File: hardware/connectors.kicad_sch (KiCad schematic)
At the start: 8 parts, among them J1 USB_C_Receptacle_USB2.0_16P, J2 FTSH-107-01-L-D-K, J3 POWER & CAN, J4 PWM1, J5 PWM2, T12 TP_VBUS

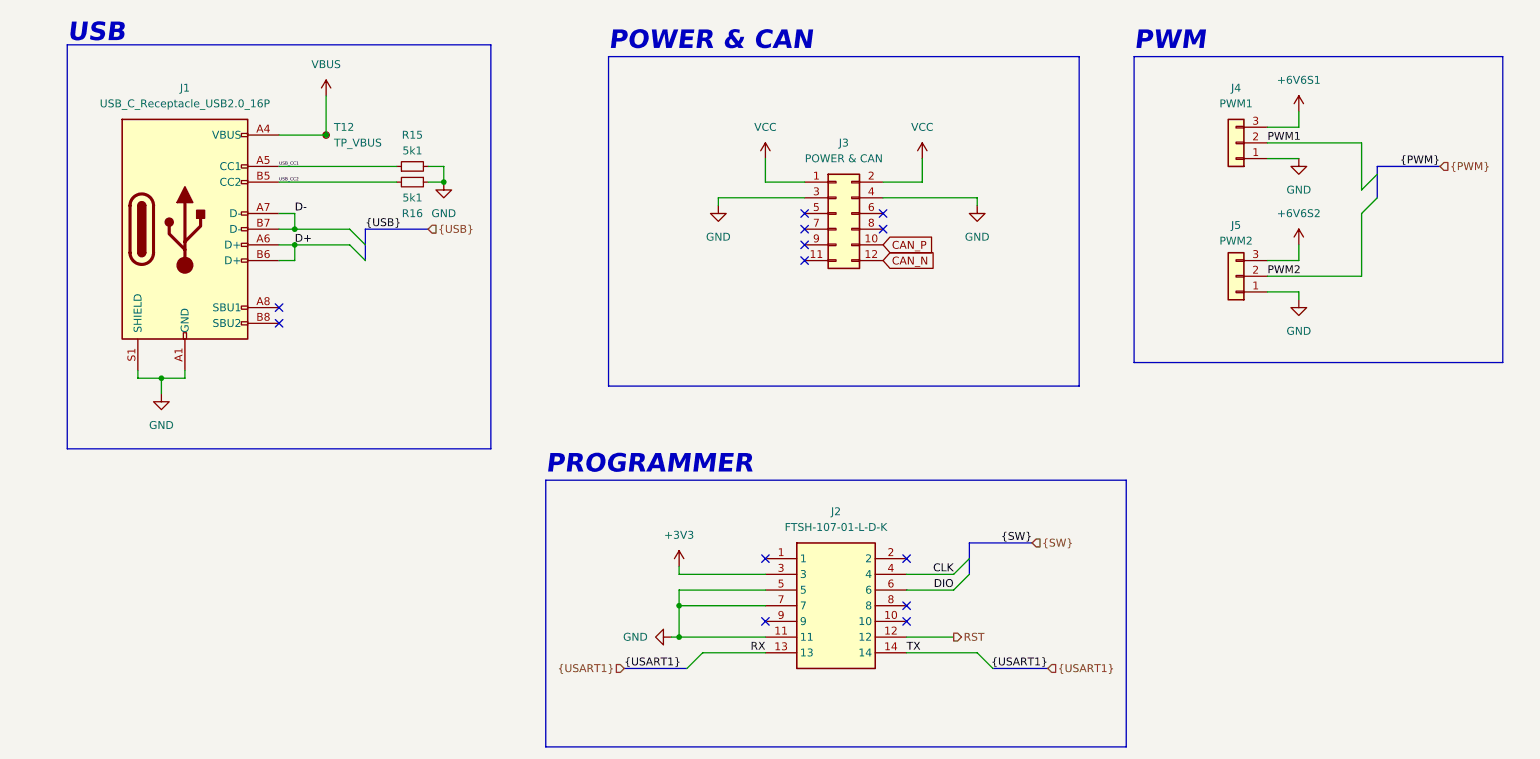
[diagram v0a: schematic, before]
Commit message: pcb & scheme update
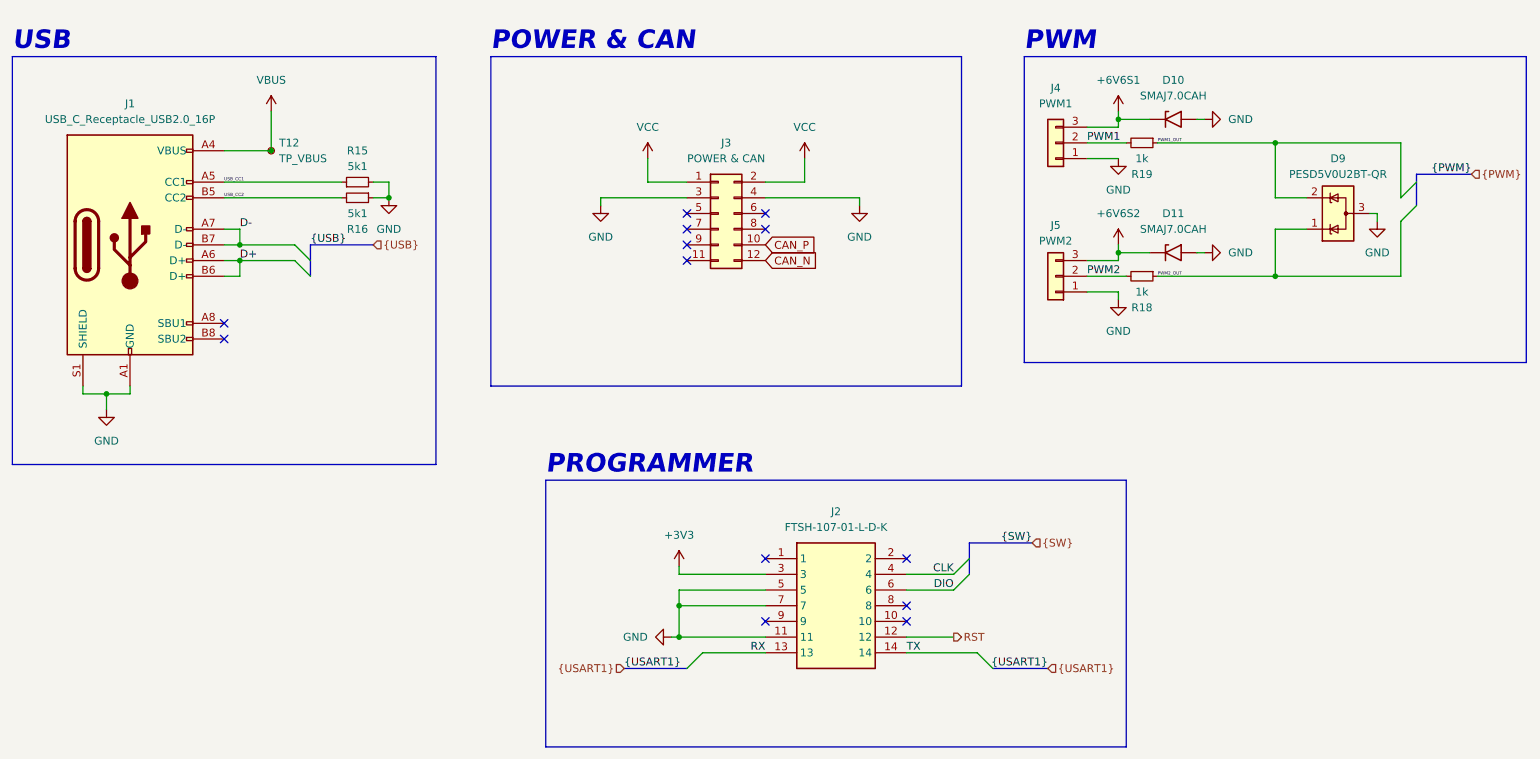
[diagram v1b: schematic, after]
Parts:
- added D10, D11: SMAJ7.0CAH, Diode_SMD:D_SMA_Handsoldering, symbol Diode:SMAJ7.0A
- added D9: PESD5V0U2BT-QR, Package_TO_SOT_SMD:SOT-23-3, symbol Power_Protection:ESDA5V3L
- added R18, R19: 1k, Resistor_SMD:R_0603_1608Metric_Pad0.98x0.95mm_HandSolder, symbol Device:R_Small
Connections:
- net +6V6S1: now also D10.1 (A1)
- net +6V6S2: now also D11.1 (A1)
- net GND: now also D10.2 (A2), D11.2 (A2), D9.3 (A)
- net PWM1: now also R19.2
- net PWM2: now also R18.2
- new net PWM1_OUT: D9.2 (K), R19.1
- new net PWM2_OUT: D9.1 (K), R18.1
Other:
- moved on the sheet: J1, J3, J4, J5, R15, R16, T12
